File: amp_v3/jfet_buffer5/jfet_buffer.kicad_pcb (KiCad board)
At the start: 2 copper layers, 40.6 x 53.3 mm, 23 parts, among them J1 PWR, J2 Conn_01x01_Pin, J3 INPUT, J4 Conn_01x01_Pin, J5 OUT1, J6 Conn_01x01_Pin, J8 OUT2, Q1 2N5457, Q2 2N5457

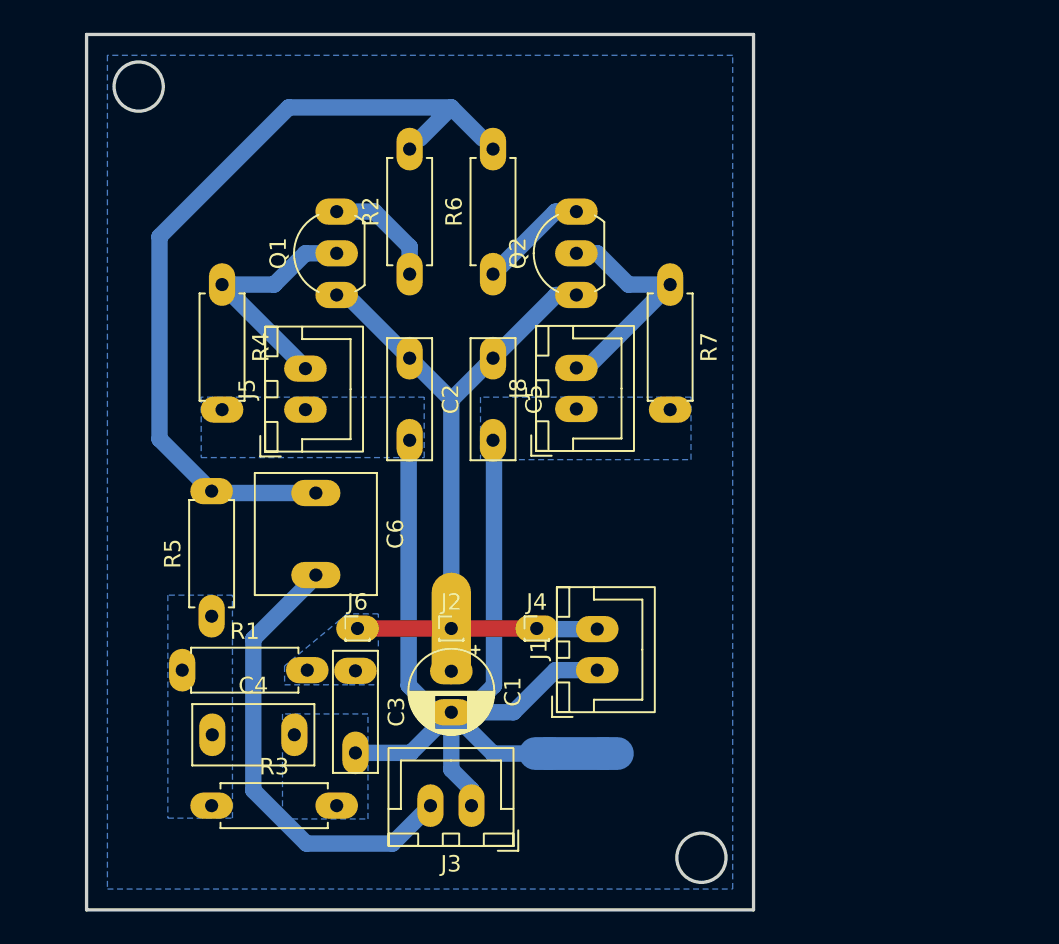
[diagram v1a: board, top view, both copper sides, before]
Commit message: updates
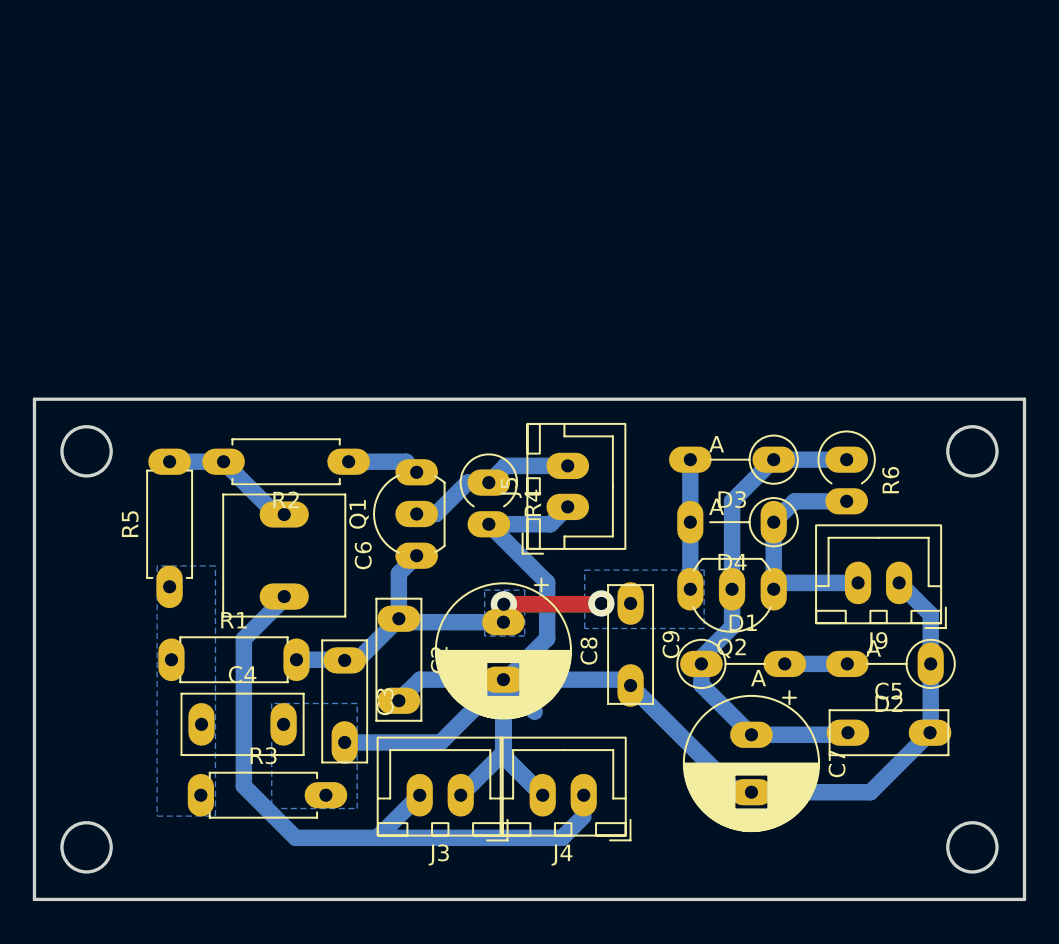
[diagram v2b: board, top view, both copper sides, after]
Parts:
- removed C1: 100uF, Capacitor_THT:CP_Radial_D5.0mm_P2.50mm
- removed J1: PWR, Connector_JST:JST_XH_B2B-XH-A_1x02_P2.50mm_Vertical
- removed J2, J6: Conn_01x01_Pin, Connector_PinHeader_1.00mm:PinHeader_1x01_P1.00mm_Vertical
- removed J8: OUT2, Connector_JST:JST_XH_B2B-XH-A_1x02_P2.50mm_Vertical
- removed R7: 3.9K, Resistor_THT:R_Axial_DIN0207_L6.3mm_D2.5mm_P7.62mm_Horizontal
- added C7: 470uF, Capacitor_THT:CP_Radial_D8.0mm_P3.50mm, F.Cu at (110.1, 90.4)
- added C8: 470uF (low ESR), Capacitor_THT:CP_Radial_D8.0mm_P3.50mm, F.Cu at (95.0, 83.6)
- added C9: 100nF, Capacitor_THT:C_Rect_L7.0mm_W2.5mm_P5.00mm, F.Cu at (102.7, 82.4)
- added D1: 1N4747, Diode_THT:D_A-405_P5.08mm_Vertical_AnodeUp, F.Cu at (107.0, 86.1)
- added D2: 1n4148, Diode_THT:D_A-405_P5.08mm_Vertical_AnodeUp, F.Cu at (121.0, 86.1)
- added D3: 1N4007, Diode_THT:D_A-405_P5.08mm_Vertical_AnodeUp, F.Cu at (111.4, 73.7)
- added D4: 1N4007, Diode_THT:D_A-405_P5.08mm_Vertical_AnodeUp, F.Cu at (111.4, 77.5)
- added J9: PWR_IN, Connector_JST:JST_XH_B2B-XH-A_1x02_P2.50mm_Vertical, F.Cu at (119.1, 81.2)
- C5: footprint Capacitor_THT:C_Rect_L7.2mm_W2.5mm_P5.00mm_FKS2_FKP2_MKS2_MKP2 -> Capacitor_THT:C_Rect_L7.0mm_W2.5mm_P5.00mm
- J3: value INPUT -> AUDIO_IN
- J4: value Conn_01x01_Pin -> AUDIO_IN; footprint Connector_PinHeader_1.00mm:PinHeader_1x01_P1.00mm_Vertical -> Connector_JST:JST_XH_B2B-XH-A_1x02_P2.50mm_Vertical
- J5: value OUT1 -> AUDIO_OUT
- NT1: footprint NetTie:NetTie-2_SMD_Pad2.0mm -> nettie 1.0:NetTie-2_SMD_Pad1.0o
- Q2: value 2N5457 -> BC549C; footprint Package_TO_SOT_THT:TO-92L_Inline_Wide -> Package_TO_SOT_THT:TO-92_Inline_Wide
- R4: footprint Resistor_THT:R_Axial_DIN0207_L6.3mm_D2.5mm_P7.62mm_Horizontal -> Resistor_THT:R_Axial_DIN0309_L9.0mm_D3.2mm_P2.54mm_Vertical
- R6: value 100 -> 240; footprint Resistor_THT:R_Axial_DIN0207_L6.3mm_D2.5mm_P7.62mm_Horizontal -> Resistor_THT:R_Axial_DIN0309_L9.0mm_D3.2mm_P2.54mm_Vertical
- moved C5 31.4 mm to (116.0, 90.3), turned to 0 degrees
- moved R6 24.3 mm to (115.9, 73.7), turned to -90 degrees
- moved Q2 21.6 mm to (111.4, 81.6), turned to 180 degrees
- moved R4 20.2 mm to (94.1, 75.1)
- moved J5 17.0 mm to (98.9, 76.5)
- moved Q1 16.6 mm to (89.7, 79.5)
- moved C2 15.9 mm to (88.6, 83.4)
- moved R2 12.0 mm to (85.5, 73.8), turned to 180 degrees
- moved J4 10.6 mm to (99.9, 94.1), turned to 180 degrees
- moved NT1 4.59 mm to (96.2, 88.3), turned to 135 degrees
- moved R5 3.13 mm to (74.6, 81.4)
- moved C6 2.33 mm to (81.6, 77.0)
- moved C3 0.91 mm to (85.3, 85.9)
- moved C4 0.91 mm to (76.6, 89.8)
- moved J3 0.91 mm to (92.4, 94.1)
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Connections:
- net /OUT1 renamed /OUT
- C2 pad 1: +20V -> /20V_JFET
- C3 pad 1: +20V -> /20V_JFET
- C5 pad 1: +20V -> Net-(D1-K)
- J4 pad 1: +20V -> /INPUT
- Q1 pad 1: +20V -> /20V_JFET
- Q2 pad 1: +20V -> /22V_REG
- Q2 pad 2: /OUT2 -> Net-(D1-K)
- Q2 pad 3: Net-(Q2-G) -> /20V_JFET
- R1 pad 2: +20V -> /20V_JFET
- R6 pad 1: Net-(Q2-G) -> Net-(D1-K)
- R6 pad 2: /VBIAS_OUT -> /22V_REG
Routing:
- net +20V: track 47.2 -> 0.00 mm
- net /VBIAS_OUT: track 49.5 -> 7.79 mm
- net /20V_JFET: track 0.00 -> 32.0 mm, vias 0 -> 2
- net Net-(D1-K): track 0.00 -> 30.9 mm
- net GND: track 66.0 -> 96.4 mm
- net /22V_REG: track 0.00 -> 14.4 mm
- net /OUT2: track 14.3 -> 0.00 mm
- net /INPUT: track 27.8 -> 38.8 mm
- net Net-(Q2-G): track 6.66 -> 0.00 mm
- net /OUT: track 15.0 -> 10.4 mm
- net Net-(D1-A): track 0.00 -> 3.81 mm
- net Net-(Q1-G): track 7.00 -> 4.41 mm
- added copper zone on B.Cu, net /20V_JFET
- removed copper zone on B.Cu, net +20V
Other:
- board size 40.6 x 53.3 mm -> 60.3 x 30.5 mm

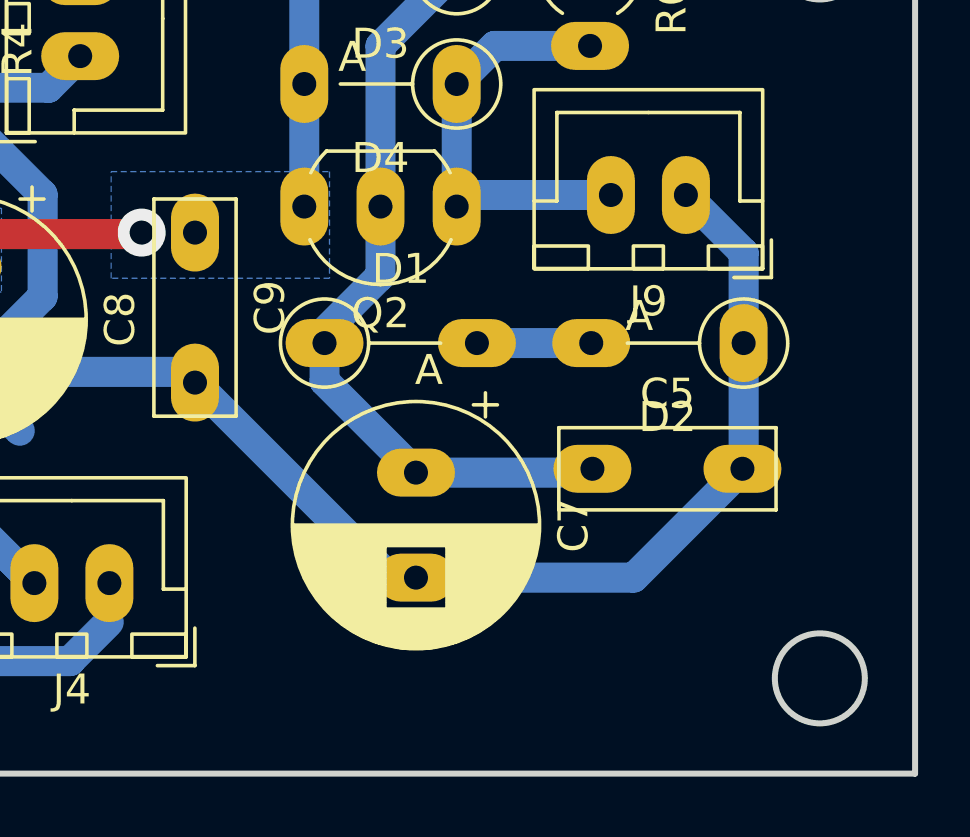
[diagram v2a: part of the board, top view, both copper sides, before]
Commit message: updates
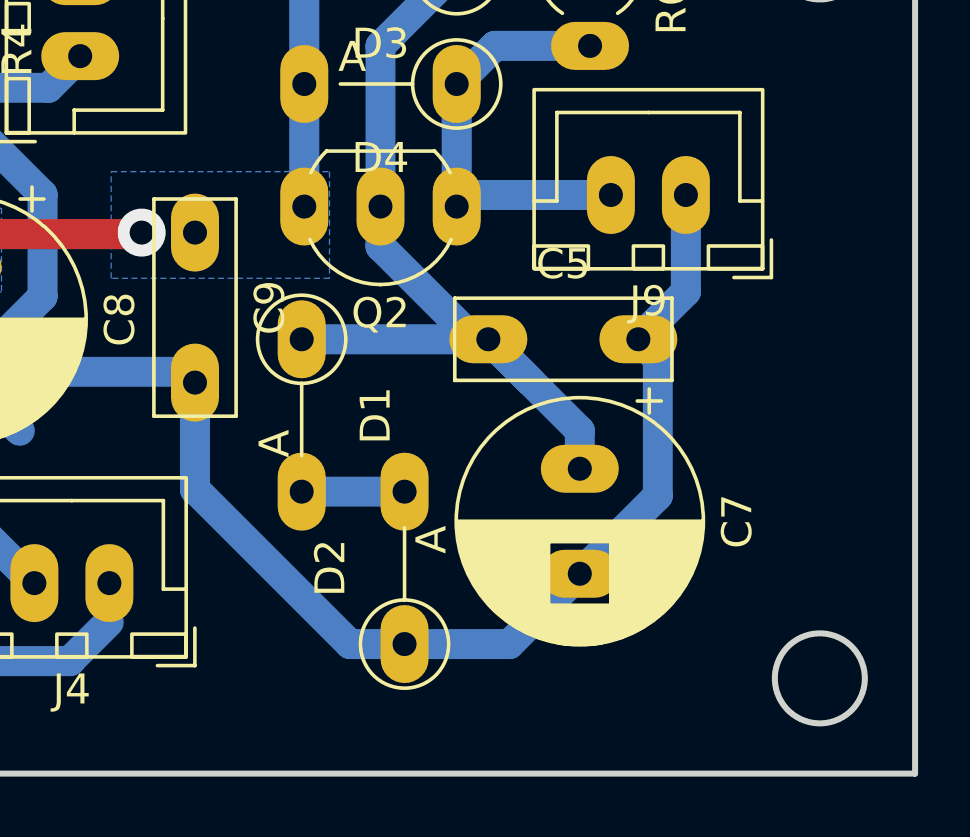
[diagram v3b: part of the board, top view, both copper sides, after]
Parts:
- moved D2 15.1 mm to (109.7, 96.1), turned to 90 degrees
- moved C5 5.54 mm to (112.5, 86.0)
- moved C7 5.46 mm to (115.5, 90.3)
- moved D1 0.77 mm to (106.3, 86.0), turned to -90 degrees
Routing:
- net GND: track 96.4 -> 101.9 mm
- net Net-(D1-K): track 30.9 -> 34.9 mm
